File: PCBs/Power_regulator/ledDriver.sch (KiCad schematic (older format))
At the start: 20 parts, among them J10 Conn_01x06_Male, J11 Conn_01x04_Male, Q1 PMOS, Q2 NMOS, Q3 Q_NMOS_GSD, Q4 Q_PMOS_GSD, Q5 Q_NMOS_GSD

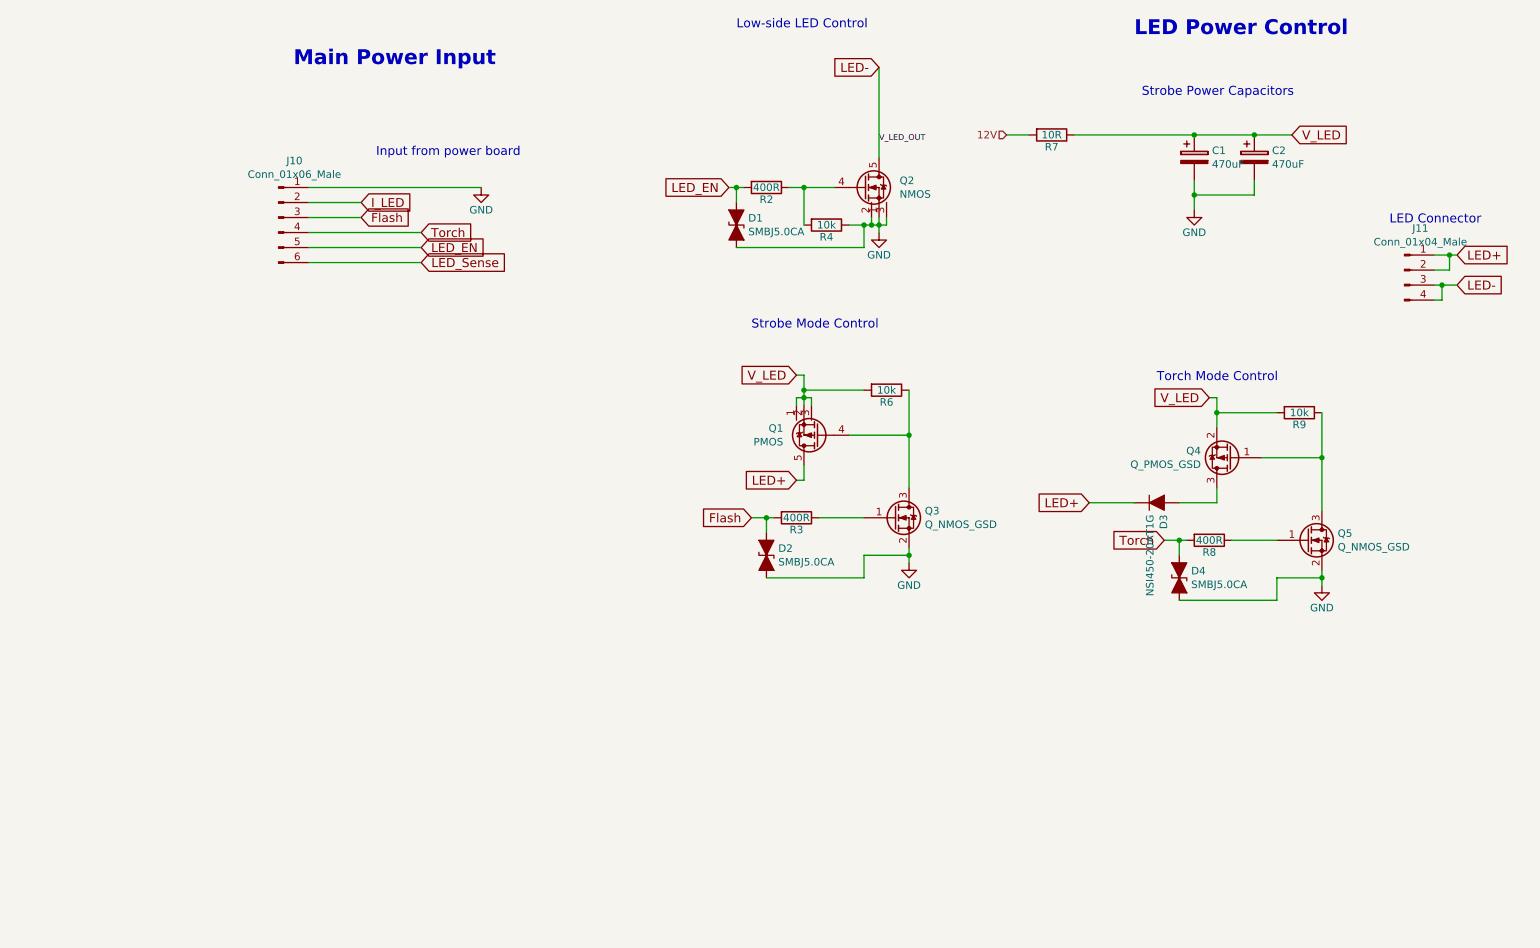
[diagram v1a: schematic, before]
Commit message: Update for revision05a
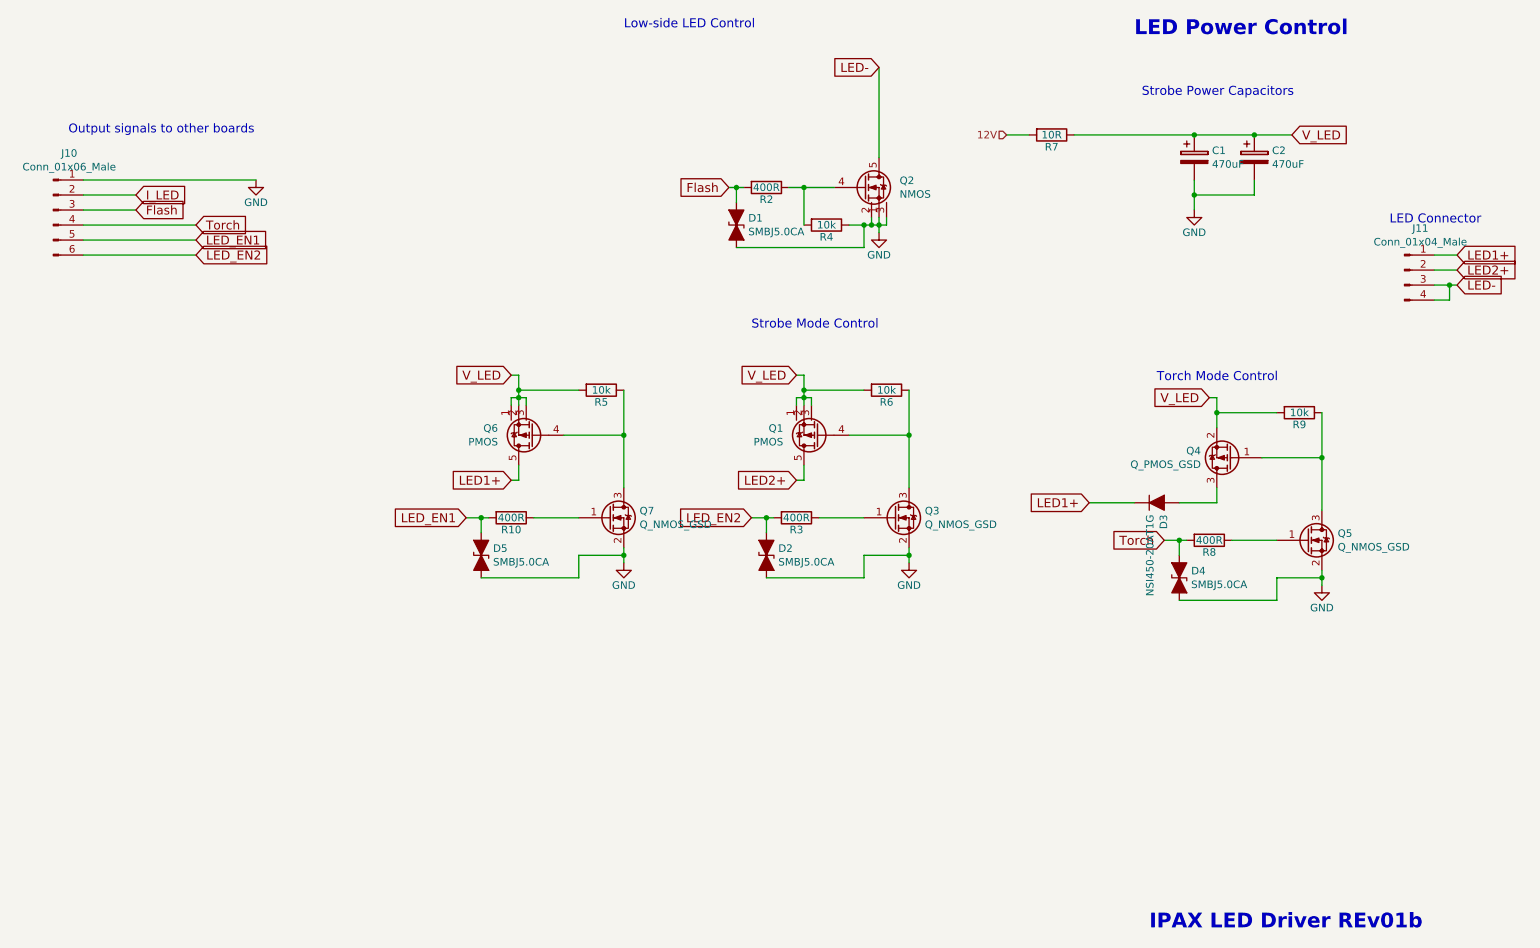
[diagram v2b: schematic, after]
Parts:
- added D5: SMBJ5.0CA, myLib:DO-214AA, symbol Device:D_TVS_ALT
- added Q6: PMOS, Package_SON:Diodes_PowerDI3333-8, symbol transistors:PMOS
- added Q7: Q_NMOS_GSD, Package_TO_SOT_SMD:SOT-23, symbol Device:Q_NMOS_GSD
- added R10: 400R, Resistor_SMD:R_0603_1608Metric, symbol Device:R
- added R5: 10k, Resistor_SMD:R_0603_1608Metric, symbol Device:R
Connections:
- net Flash: now also D1.1 (A1), R2.2; no longer D2.1 (A1), R3.2
- net GND: now also D5.2 (A2), Q7.2 (S)
- net V_LED: now also Q6.1 (S), Q6.2 (S), Q6.3 (S), R5.2
- net LED+ renamed LED1+
- net LED1+: now also Q6.5 (D); no longer J11.2 (Pin_2), Q1.5 (D)
- removed net LED_EN: D1.1 (A1), J10.5 (Pin_5), R2.2
- net LED_Sense renamed LED_EN2
- net LED_EN2: now also D2.1 (A1), R3.2
- new net: Q7.1 (G), R10.1
- new net: Q6.4 (G), Q7.3 (D), R5.1
- new net LED2+: J11.2 (Pin_2), Q1.5 (D)
- new net LED_EN1: D5.1 (A1), J10.5 (Pin_5), R10.2
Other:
- note added: "IPAX LED Driver REv01b"
- note added: "Output signals to other boards"
- note removed: "Input from power board"
- note removed: "Main Power Input"
- moved on the sheet: J10
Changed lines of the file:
@@
 Comment4 ""
 $EndDescr
+Text Notes 8250 6900 0    98   ~ 20
+IPAX LED Driver REv01b
 $Comp
 L Device:R R?
@@
 Text Notes 8200 1350 0    60   ~ 0
 Strobe Power Capacitors
-Text GLabel 5600 4150 0    60   Input ~ 0
+Text GLabel 5450 1950 0    60   Input ~ 0
 Flash
 $Comp
@@
 V_LED
 Text GLabel 5900 3900 0    60   Input ~ 0
-LED+
+LED2+
 $Comp
 L power:GND #PWR?
@@
 $EndComp
 Text GLabel 10300 2400 2    60   Input ~ 0
-LED+
+LED1+
 Text GLabel 10300 2600 2    60   Input ~ 0
 LED-
@@
 Torch Mode Control
 Text GLabel 7850 4050 0    60   Input ~ 0
-LED+
+LED1+
 $Comp
 L power:GND #PWR?
@@
 Wire Wire Line
 	5950 1950 6150 1950
-Text GLabel 5450 1950 0    60   Input ~ 0
-LED_EN
+Text GLabel 5600 4150 0    60   Input ~ 0
+LED_EN2
 Wire Wire Line
 	5450 1950 5500 1950
-Text Notes 5500 900  0    60   ~ 0
+Text Notes 4750 900  0    60   ~ 0
 Low-side LED Control
 $Comp
@@
 Wire Wire Line
 	6350 2200 6400 2200
-Text Label 6450 1650 0    39   ~ 0
-V_LED_OUT
-Wire Wire Line
-	3000 2050 2650 2050
-Wire Wire Line
-	3000 2150 2650 2150
-Text GLabel 3000 2050 2    59   Input ~ 0
+Wire Wire Line
+	1500 2000 1150 2000
+Wire Wire Line
+	1500 2100 1150 2100
+Text GLabel 1500 2000 2    59   Input ~ 0
 I_LED
-Text GLabel 3000 2150 2    59   Input ~ 0
+Text GLabel 1500 2100 2    59   Input ~ 0
 Flash
-Text Notes 3100 1750 0    59   ~ 0
-Input from power board
-Wire Wire Line
-	2650 2350 3400 2350
-Wire Wire Line
-	2650 2250 3400 2250
-Wire Wire Line
-	2650 1950 3800 1950
-Text GLabel 3400 2350 2    59   Input ~ 0
-LED_EN
-Text GLabel 3400 2250 2    59   Input ~ 0
+Text Notes 1050 1600 0    59   ~ 0
+Output signals to other boards
+Wire Wire Line
+	1150 2300 1900 2300
+Wire Wire Line
+	1150 2200 1900 2200
+Wire Wire Line
+	1150 1900 2300 1900
+Text GLabel 1900 2300 2    59   Input ~ 0
+LED_EN1
+Text GLabel 1900 2200 2    59   Input ~ 0
 Torch
 $Comp
 L power:GND #PWR?
 U 1 1 5C475009
-P 3800 1950
+P 2300 1900
 AR Path="/5BC9CFF4/5C475009" Ref="#PWR?"  Part="1"
 AR Path="/5988C2E9/5C475009" Ref="#PWR?"  Part="1"
 AR Path="/5C475009" Ref="#PWR?"  Part="1"
 AR Path="/5D134CF5/5C475009" Ref="#PWR0111"  Part="1"
-F 0 "#PWR0111" H 3800 1700 50  0001 C CNN
-F 1 "GND" H 3800 1800 50  0000 C CNN
-F 2 "" H 3800 1950 50  0000 C CNN
-F 3 "" H 3800 1950 50  0000 C CNN
-	1    3800 1950
+F 0 "#PWR0111" H 2300 1650 50  0001 C CNN
+F 1 "GND" H 2300 1750 50  0000 C CNN
+F 2 "" H 2300 1900 50  0000 C CNN
+F 3 "" H 2300 1900 50  0000 C CNN
+	1    2300 1900
 	1    0    0    -1
 $EndComp
@@
 L Connector:Conn_01x06_Male J10
 U 1 1 5C460366
-P 2450 2150
-F 0 "J10" H 2556 2528 50  0000 C CNN
-F 1 "Conn_01x06_Male" H 2556 2437 50  0000 C CNN
-F 2 "myLib:conn_1x06_1.5mm" H 2450 2150 50  0001 C CNN
-F 3 "~" H 2450 2150 50  0001 C CNN
-	1    2450 2150
-	1    0    0    -1
-$EndComp
-Text Notes 2550 1150 0    99   ~ 20
-Main Power Input
+P 950 2100
+F 0 "J10" H 1056 2478 50  0000 C CNN
+F 1 "Conn_01x06_Male" H 1056 2387 50  0000 C CNN
+F 2 "myLib:conn_1x06_1.5mm" H 950 2100 50  0001 C CNN
+F 3 "~" H 950 2100 50  0001 C CNN
+	1    950  2100
+	1    0    0    -1
+$EndComp
 $Comp
 L Device:CP C1
@@
 Wire Wire Line
 	8950 1600 9200 1600
-Text GLabel 3400 2450 2    60   Input ~ 0
-LED_Sense
-Wire Wire Line
-	3400 2450 2650 2450
+Text GLabel 1900 2400 2    60   Input ~ 0
+LED_EN2
+Wire Wire Line
+	1900 2400 1150 2400
 $Comp
 L transistors:NMOS Q2
@@
 	1    0    0    -1
 $EndComp
-Wire Wire Line
-	10150 2400 10250 2400
-Wire Wire Line
-	10150 2500 10250 2500
-Wire Wire Line
-	10250 2500 10250 2400
-Connection ~ 10250 2400
-Wire Wire Line
-	10250 2400 10300 2400
-Wire Wire Line
-	10300 2600 10200 2600
-Wire Wire Line
-	10150 2700 10200 2700
-Wire Wire Line
-	10200 2700 10200 2600
-Connection ~ 10200 2600
-Wire Wire Line
-	10200 2600 10150 2600
 $Comp
 L Device:Q_PMOS_GSD Q4
@@
 Wire Wire Line
 	6450 1150 6450 1750
+Wire Wire Line
+	10150 2600 10250 2600
+$Comp
+L Device:R R?
+U 1 1 5E69900E
+P 4000 4150
+AR Path="/5BC9CFF4/5E69900E" Ref="R?"  Part="1"
+AR Path="/5988C2E9/5E69900E" Ref="R?"  Part="1"
+AR Path="/5E69900E" Ref="R?"  Part="1"
+AR Path="/5D134CF5/5E69900E" Ref="R10"  Part="1"
+F 0 "R10" V 4080 4150 50  0000 C CNN
+F 1 "400R" V 4000 4150 50  0000 C CNN
+F 2 "Resistor_SMD:R_0603_1608Metric" V 3930 4150 50  0001 C CNN
+F 3 "" H 4000 4150 50  0000 C CNN
+	1    4000 4150
+	0    1    1    0
+$EndComp
+$Comp
+L Device:R R?
+U 1 1 5E699014
+P 4600 3300
+AR Path="/5BC9CFF4/5E699014" Ref="R?"  Part="1"
+AR Path="/5988C2E9/5E699014" Ref="R?"  Part="1"
+AR Path="/5E699014" Ref="R?"  Part="1"
+AR Path="/5D134CF5/5E699014" Ref="R5"  Part="1"
+F 0 "R5" V 4680 3300 50  0000 C CNN
+F 1 "10k" V 4600 3300 50  0000 C CNN
+F 2 "Resistor_SMD:R_0603_1608Metric" V 4530 3300 50  0001 C CNN
+F 3 "" H 4600 3300 50  0000 C CNN
+	1    4600 3300
+	0    1    1    0
+$EndComp
+Wire Wire Line
+	3700 4150 3800 4150
+Text GLabel 4000 3200 0    60   Input ~ 0
+V_LED
+Text GLabel 4000 3900 0    60   Input ~ 0
+LED1+
+$Comp
+L power:GND #PWR?
+U 1 1 5E69901D
+P 4750 4450
+AR Path="/5BC9CFF4/5E69901D" Ref="#PWR?"  Part="1"
+AR Path="/5988C2E9/5E69901D" Ref="#PWR?"  Part="1"
+AR Path="/5E69901D" Ref="#PWR?"  Part="1"
+AR Path="/5D134CF5/5E69901D" Ref="#PWR0113"  Part="1"
+F 0 "#PWR0113" H 4750 4200 50  0001 C CNN
+F 1 "GND" H 4750 4300 50  0000 C CNN
+F 2 "" H 4750 4450 50  0000 C CNN
+F 3 "" H 4750 4450 50  0000 C CNN
+	1    4750 4450
+	1    0    0    -1
+$EndComp
+Text GLabel 3700 4150 0    60   Input ~ 0
+LED_EN1
+$Comp
+L Device:D_TVS_ALT D5
+U 1 1 5E699024
+P 3800 4400
+F 0 "D5" V 3754 4479 50  0000 L CNN
+F 1 "SMBJ5.0CA" V 3845 4479 50  0000 L CNN
+F 2 "myLib:DO-214AA" H 3800 4400 50  0001 C CNN
+F 3 "~" H 3800 4400 50  0001 C CNN
+	1    3800 4400
+	0    1    1    0
+$EndComp
+Wire Wire Line
+	3800 4250 3800 4150
+Connection ~ 3800 4150
+Wire Wire Line
+	3800 4150 3850 4150
+$Comp
+L transistors:PMOS Q6
+U 1 1 5E69902D
+P 4150 3600
+F 0 "Q6" H 4388 3554 50  0000 L CNN
+F 1 "PMOS" H 4388 3645 50  0000 L CNN
+F 2 "Package_SON:Diodes_PowerDI3333-8" H 4350 3525 50  0001 L CIN
+F 3 "http://www.vishay.com/docs/70209/70209.pdf" H 4150 3600 50  0001 L CNN
+	1    4150 3600
+	-1   0    0    1
+$EndComp
+$Comp
+L Device:Q_NMOS_GSD Q7
+U 1 1 5E699033
+P 4650 4150
+F 0 "Q7" H 4855 4196 50  0000 L CNN
+F 1 "Q_NMOS_GSD" H 4855 4105 50  0000 L CNN
+F 2 "Package_TO_SOT_SMD:SOT-23" H 4850 4250 50  0001 C CNN
+F 3 "~" H 4650 4150 50  0001 C CNN
+	1    4650 4150
+	1    0    0    -1
+$EndComp
+Wire Wire Line
+	4000 3200 4050 3200
+Wire Wire Line
+	4050 3200 4050 3300
+Wire Wire Line
+	4000 3400 4000 3350
+Wire Wire Line
+	4000 3350 4050 3350
+Connection ~ 4050 3350
+Wire Wire Line
+	4050 3350 4050 3400
+Wire Wire Line
+	4100 3400 4100 3350
+Wire Wire Line
+	4100 3350 4050 3350
+Wire Wire Line
+	4050 3800 4050 3900
+Wire Wire Line
+	4050 3900 4000 3900
+Wire Wire Line
+	4450 3300 4050 3300
+Connection ~ 4050 3300
+Wire Wire Line
+	4050 3300 4050 3350
+Wire Wire Line
+	4750 3950 4750 3600
+Wire Wire Line
+	4350 3600 4750 3600
+Connection ~ 4750 3600
+Wire Wire Line
+	4750 3600 4750 3300
+Wire Wire Line
+	4150 4150 4450 4150
+Wire Wire Line
+	4750 4350 4750 4400
+Wire Wire Line
+	3800 4550 4450 4550
+Wire Wire Line
+	4450 4550 4450 4400
+Wire Wire Line
+	4450 4400 4750 4400
+Connection ~ 4750 4400
+Wire Wire Line
+	4750 4400 4750 4450
+Wire Wire Line
+	10150 2700 10250 2700
+Wire Wire Line
+	10250 2700 10250 2600
+Connection ~ 10250 2600
+Wire Wire Line
+	10250 2600 10300 2600
+Wire Wire Line
+	10150 2400 10300 2400
+Text GLabel 10300 2500 2    60   Input ~ 0
+LED2+
+Wire Wire Line
+	10150 2500 10300 2500
 $EndSCHEMATC
